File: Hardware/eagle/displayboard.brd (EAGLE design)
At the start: 70.8 x 45.7 mm, 11 parts, among them J1 CON_HEADER_1X08-SMD, J2 FH12-10S-0.5SH, J3 CON_HEADER_1X08-SMD

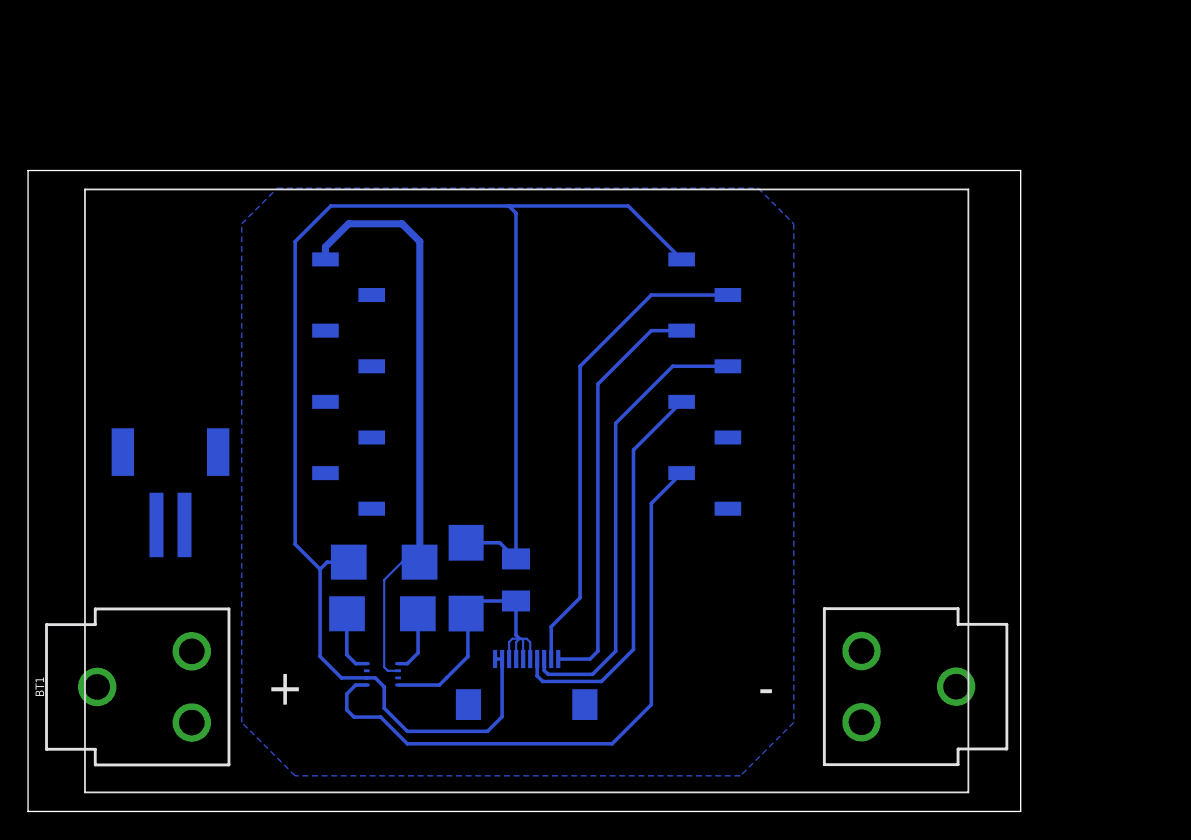
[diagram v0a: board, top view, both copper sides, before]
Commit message: Update to board design
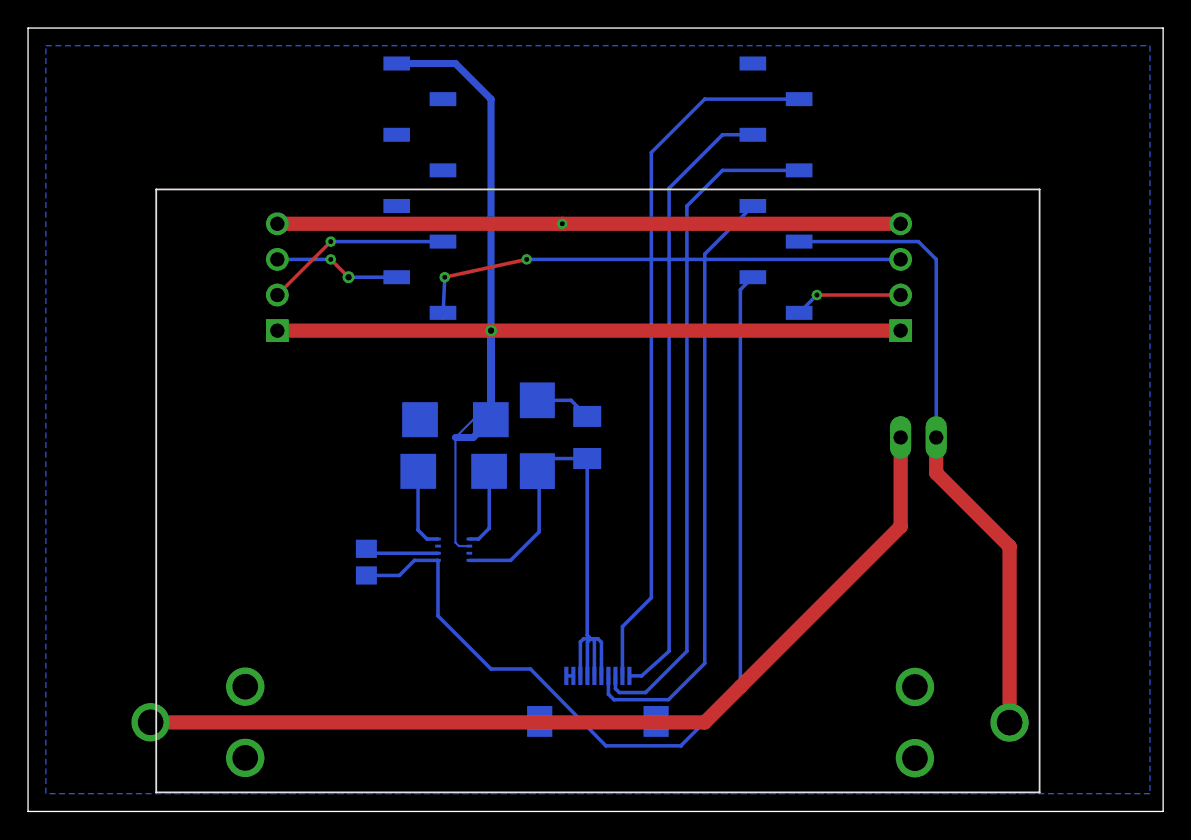
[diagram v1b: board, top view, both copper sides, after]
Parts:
- added I2C, UART: CON_HEADER_1X04, dp_devices.v6:M1X4
- added R1: 100k, rcl:R0805
- CN1: device adafruit:JST-PH-2-SMT-RA -> pinhead:1X02
- moved CN1 53.4 mm to (63.5, 26.7), turned to 180 degrees
- moved J1 14.9 mm to (53.3, 44.5)
- moved J3 14.9 mm to (27.9, 44.5)
- moved C1 11.4 mm to (30.4, 24.3)
- moved C2 11.4 mm to (36.3, 26.8)
- moved C3 11.4 mm to (30.5, 27.9)
- moved C4 11.4 mm to (39.9, 26.7)
- moved U$1 10.2 mm to (30.4, 18.7)
- moved J2 5.22 mm to (40.6, 6.42)
- moved U$2 5.08 mm to (40.6, 22.9)
- moved BT1 4.58 mm to (39.4, 6.35), flipped to the bottom
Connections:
- removed net N$12: J3.6
- removed net N$13: J3.7
- removed net N$14: J3.8
- removed net N$3: BT1.PWR@1, CN1.1
- removed net N$8: J1.8
- new net RX: J3.7, UART.3
- new net SCL: I2C.2, J1.8
- new net SDA: I2C.3, J3.8
- new net TX: J3.6, UART.2
- new net V+: BT1.PWR@1, CN1.2, J1.6
- net DISP_EN: now also R1.1
- net GND: now also I2C.4, R1.2, UART.4
- net N$5: now also CN1.1; no longer CN1.2
- net VCC: now also I2C.1, UART.1
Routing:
- net N$5: track 0.00 -> 65.6 mm
- net GND: track 113.3 -> 54.4 mm, vias 0 -> 1
- net VCC: track 42.1 -> 96.2 mm, vias 0 -> 1
- net V+: track 0.00 -> 45.5 mm
- net SDA: track 0.00 -> 36.0 mm, vias 0 -> 2
- net DISP_EN: track 44.1 -> 66.3 mm
- net VDD: track 22.8 -> 40.2 mm
- net MOSI: track 34.4 -> 50.3 mm
- net CS: track 32.7 -> 48.2 mm
- net EXTCOM: track 28.3 -> 43.5 mm
- net SCLK: track 29.7 -> 44.1 mm
- net TX: track 0.00 -> 13.4 mm, vias 0 -> 1
- net RX: track 0.00 -> 9.04 mm, vias 0 -> 2
- net SCL: track 0.00 -> 7.77 mm, vias 0 -> 1
- net N$2: track 4.54 -> 5.81 mm
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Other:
- board size 70.8 x 45.7 mm -> 81 x 55.9 mm
- board text added: "+"
- board text added: "-"
- board text added: "A Hack-A-Gecko project"
- board text added: "Meeting Room Monitor"
- board text added: "RX"
- board text added: "SCL"
- board text added: "SDA"
- board text added: "TX"
- board text added: "by Steven Cooreman"
